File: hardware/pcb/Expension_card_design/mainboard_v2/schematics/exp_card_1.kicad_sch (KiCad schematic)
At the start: 6 parts, among them J1 528850374

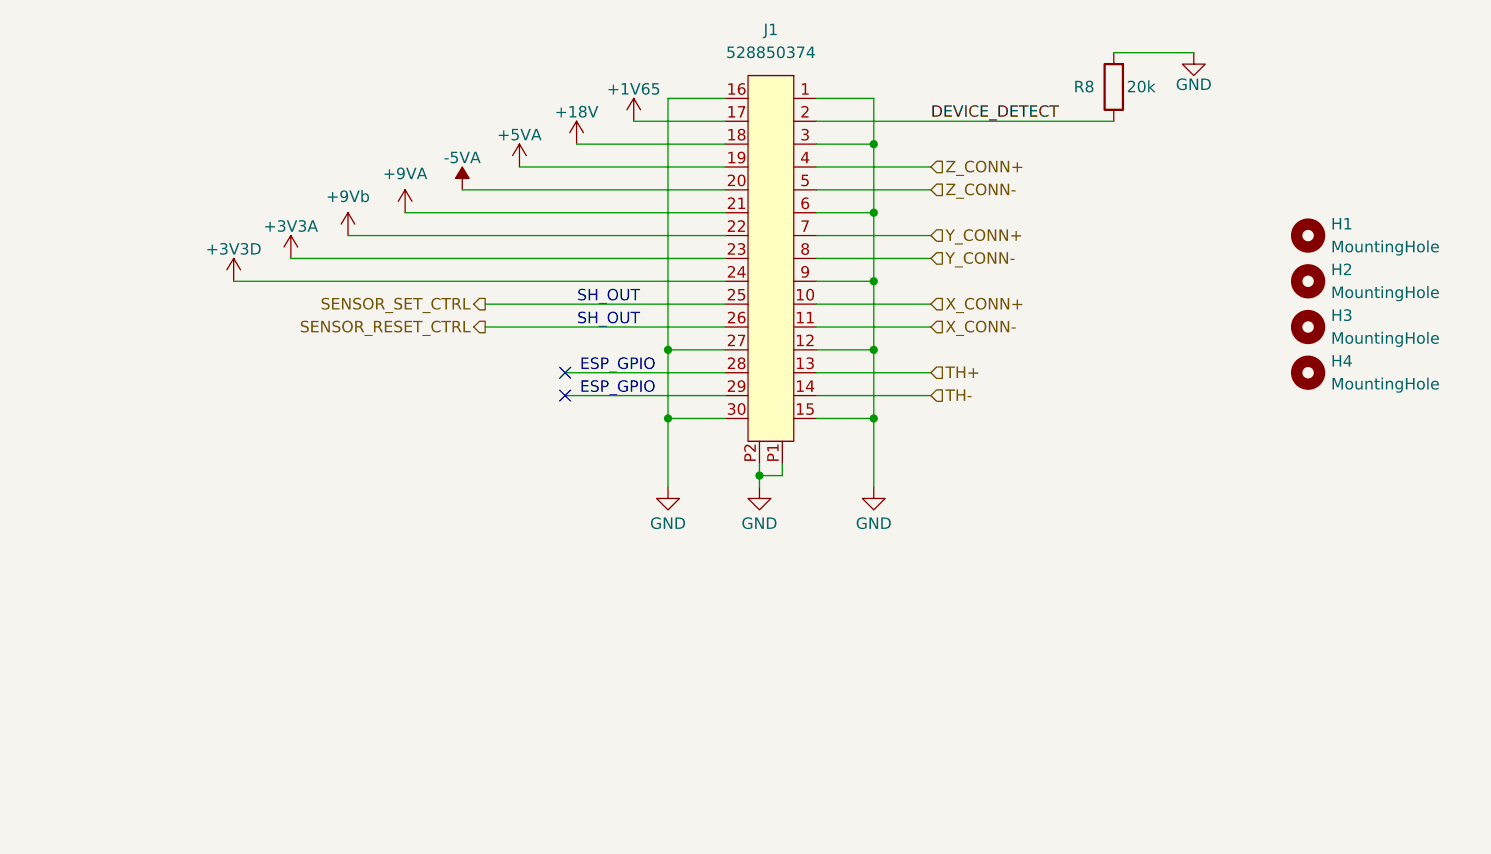
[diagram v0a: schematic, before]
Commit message: kicad mag board done
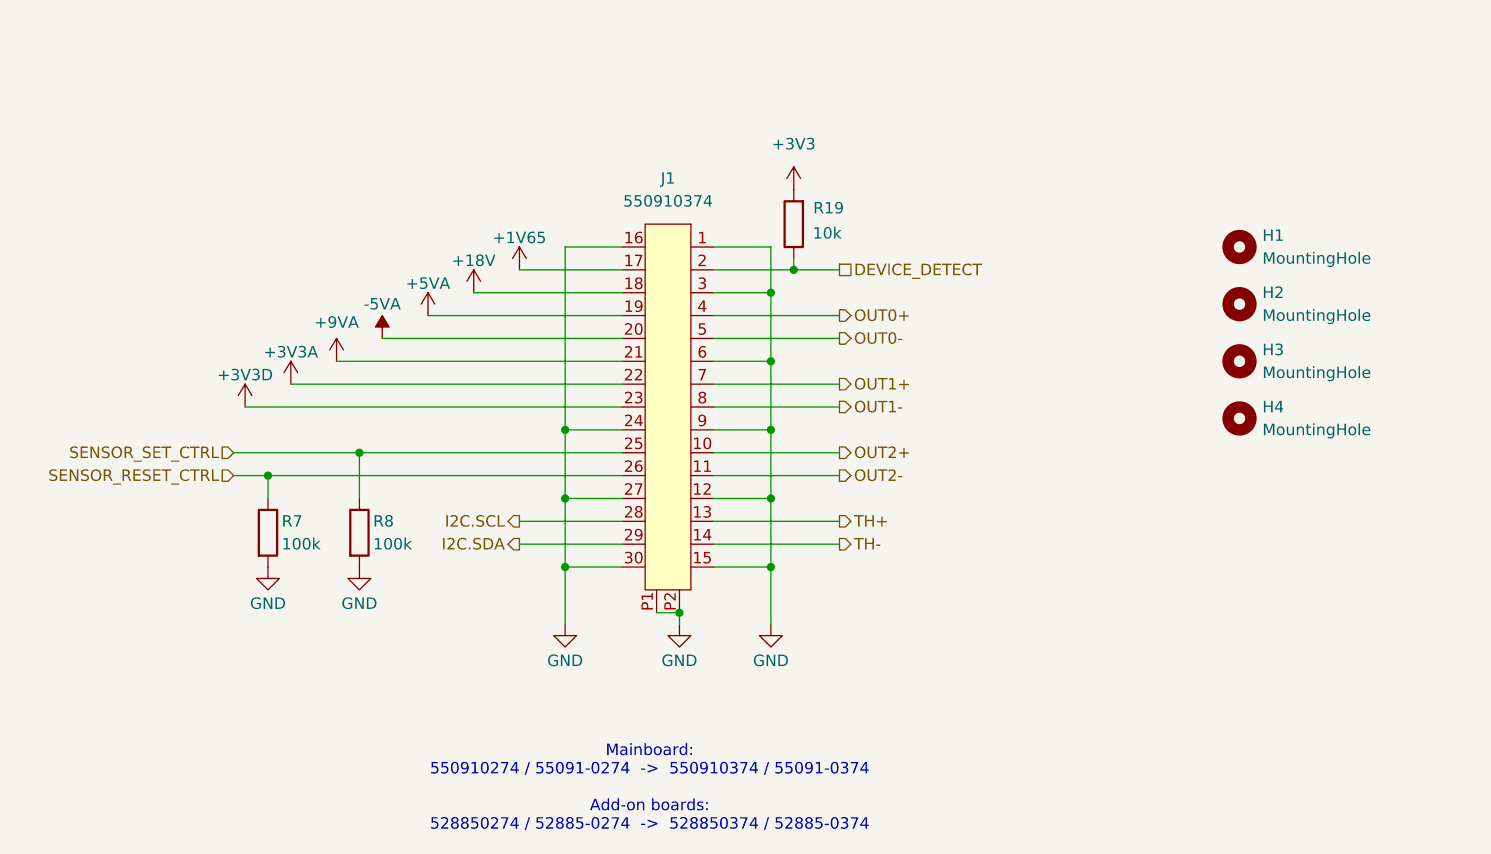
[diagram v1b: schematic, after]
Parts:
- removed J1: 528850374, magnode_footprints:CONN_MOLEX_02x15_52885-0374, symbol magnode_symbols:52885-0374
- added J1: 550910374, magnode_footprints:CONN_MOLEX_02x15_55091-0374, symbol magnode_symbols:55091-0374
- added R19: 10k, Resistor_SMD:R_0603_1608Metric, symbol Device:R
- added R7: 100k, Resistor_SMD:R_0603_1608Metric, symbol Device:R
- R8: value 20k -> 100k; LCSC C4184 -> C25803
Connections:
- net +18V: now also J1.18
- net +1V65: now also J1.17
- net +3V3A: now also J1.22
- net +3V3D: now also J1.23
- net +5VA: now also J1.19
- net +9VA: now also J1.21
- net -5VA: now also J1.20
- net DEVICE_DETECT: now also J1.2, R19.1; no longer R8.1
- net GND: now also J1.1, J1.12, J1.15, J1.16, J1.24, J1.27, J1.3, J1.30, J1.6, J1.9, J1.P1, J1.P2, R7.2
- net SENSOR_RESET_CTRL: now also J1.26, R7.1
- net SENSOR_SET_CTRL: now also R8.1, J1.25
- net TH+: now also J1.13
- net TH-: now also J1.14
- new net +3V3: R19.2
- new net I2C.SCL: J1.28
- new net I2C.SDA: J1.29
- new net OUT0+: J1.4
- new net OUT0-: J1.5
- new net OUT1+: J1.7
- new net OUT1-: J1.8
- new net OUT2+: J1.10
- new net OUT2-: J1.11
- no-connect marks 2 -> 0
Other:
- note added: "Mainboard: 550910274 / 55091-0274 -> 550910374 / 55091-0374 Add-on boards: 528850274 / 52885-0274 -> 528850374 / 52885-0374"
- note removed: "ESP_GPIO"
- note removed: "SH_OUT"
